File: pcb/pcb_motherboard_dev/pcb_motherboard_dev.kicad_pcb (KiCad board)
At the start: 4 copper layers, 100 x 100 mm, 176 parts, among them J1 Screw_Terminal_01x02, J13 LED, J2 Conn_01x04_Male, J4 Conn_02x04_Odd_Even, J5 AudioJack3, J6 SYNC, J7 Conn_02x13_Odd_Even, J8 Micro_SD_Card, Q1 DMG9926USD, Q2 IRF7410TRPBF, Q3 IRLML2244TRPBF, Q4 BSS806NE, Q5 BSS806NE, Q6 IRF7410TRPBF, Q7 BSS806NE, SW1 SW_Push, SW2 SW_DIP_x01, SW3 SW_DIP_x01, U1 TP4056, U10 FT232breakout, U11 DS18B20Z, U12 2POS_JUMPER_8BIT, U13 DS18B20Z, U2 LP38501, U3 TP4056withprotect, U4 NT1713C, U5 EL357NC, U6 EL357NC, U7 74HC165, U8 ESP32-WROOM-32, U9 MCP6002-xSN, Y1 32.768 kHz

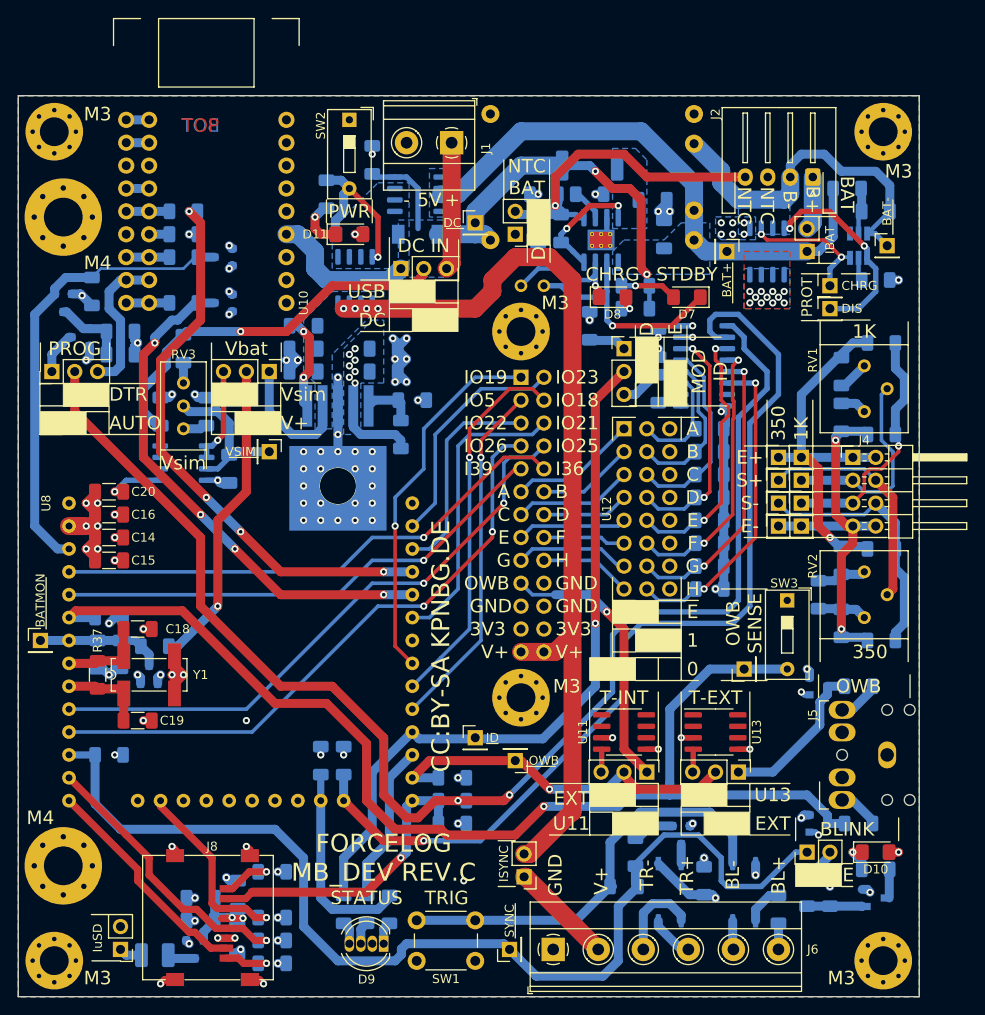
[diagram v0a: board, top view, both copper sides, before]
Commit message: CleanUp
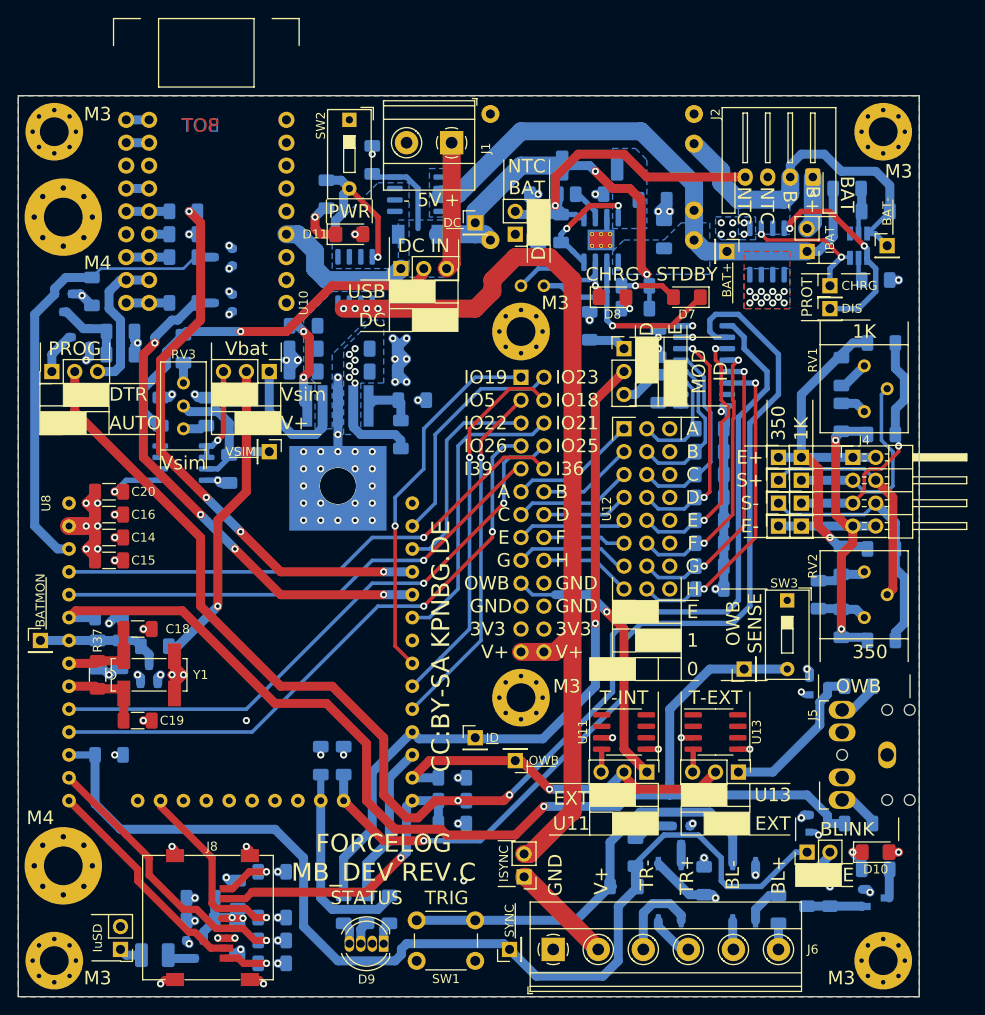
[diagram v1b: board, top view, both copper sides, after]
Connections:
- net /CONTROLLER/IO_5|V~CS renamed /CONTROLLER/IO_5|V~{CS}
- net /POWER/~LED_CHRG renamed /POWER/~{LED_CHRG}
- net /POWER/~LED_STBY renamed /POWER/~{LED_STBY}
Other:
- net class Default removed
